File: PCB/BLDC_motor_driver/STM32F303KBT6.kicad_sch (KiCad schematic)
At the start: 3 parts, among them U2 AS5048A, U7 STM32F303K8Tx, U8 SN65HVD230

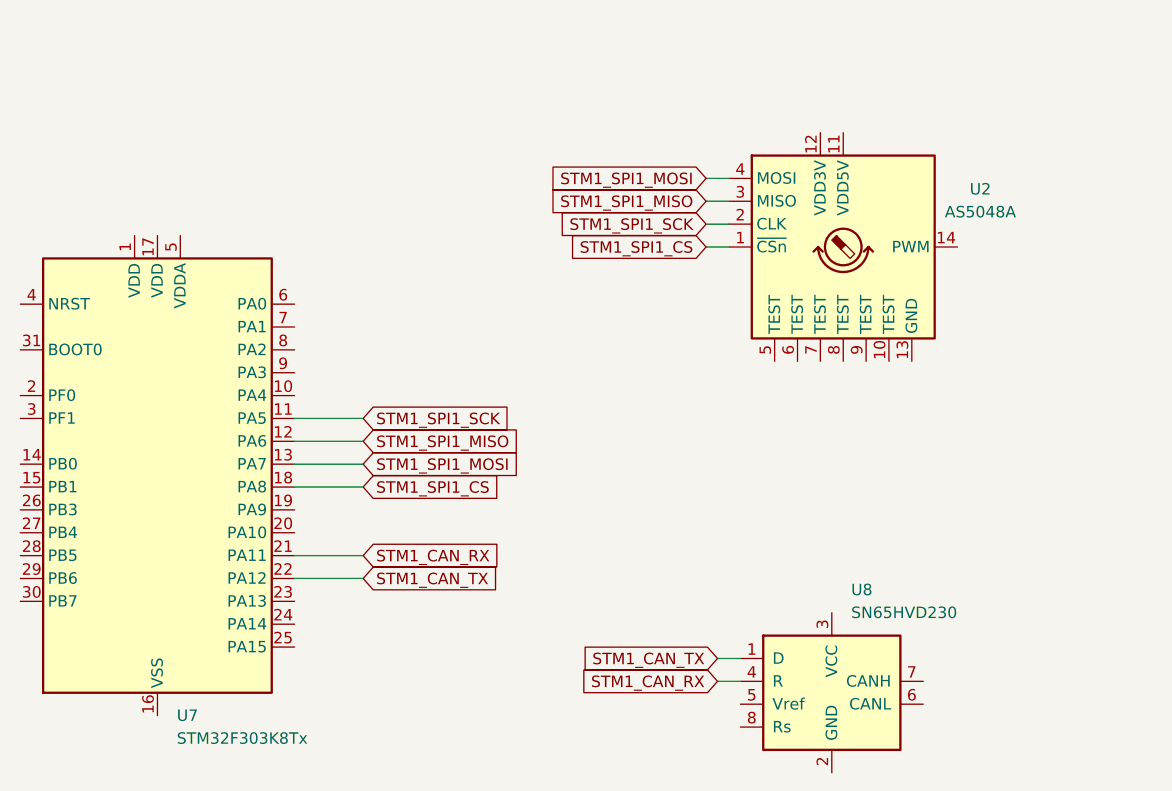
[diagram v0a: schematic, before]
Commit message: updated schematic
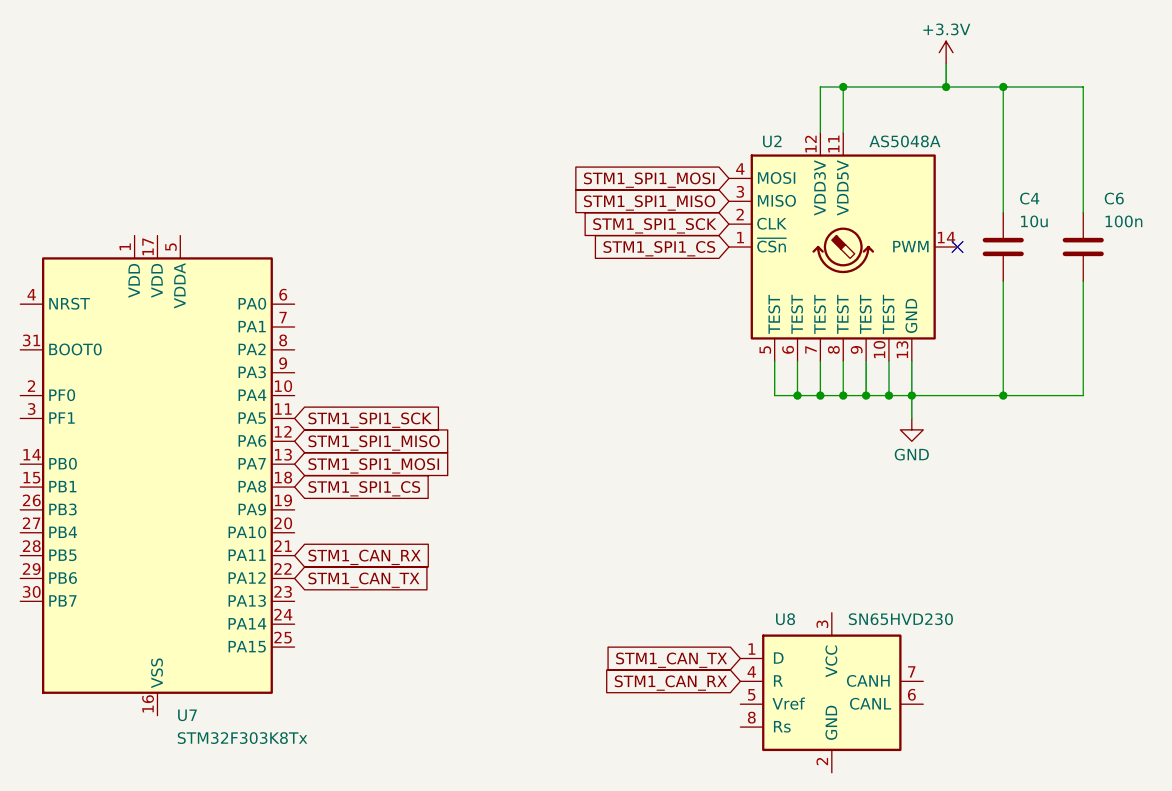
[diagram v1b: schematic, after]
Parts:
- added C4: 10u, Capacitor_SMD:C_0504_1310Metric, symbol Device:C
- added C6: 100n, Capacitor_SMD:C_0504_1310Metric, symbol Device:C
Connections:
- net GND: now reaches U2.10 (TEST)
- net GND: now also U2.13 (GND), U2.5 (TEST), U2.6 (TEST), U2.7 (TEST), U2.8 (TEST), U2.9 (TEST), C4.2, C6.2
- net +3.3V: now reaches U2.11 (VDD5V)
- net +3.3V: now also U2.12 (VDD3V), C4.1, C6.1
- no-connect marks 0 -> 1
